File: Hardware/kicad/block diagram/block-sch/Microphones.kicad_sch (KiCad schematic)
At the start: 37 parts, among them J18 Conn_01x03, J19 Conn_01x03, J20 AudioJack3, K3 G6K-2, K4 G6K-2, Q3 BC817, U21 LM833D

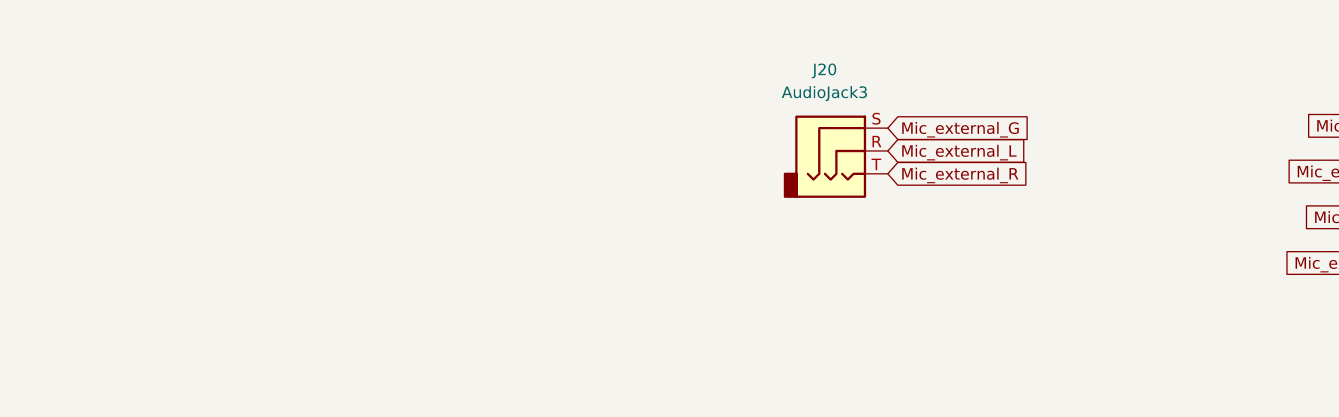
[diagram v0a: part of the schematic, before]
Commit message: new
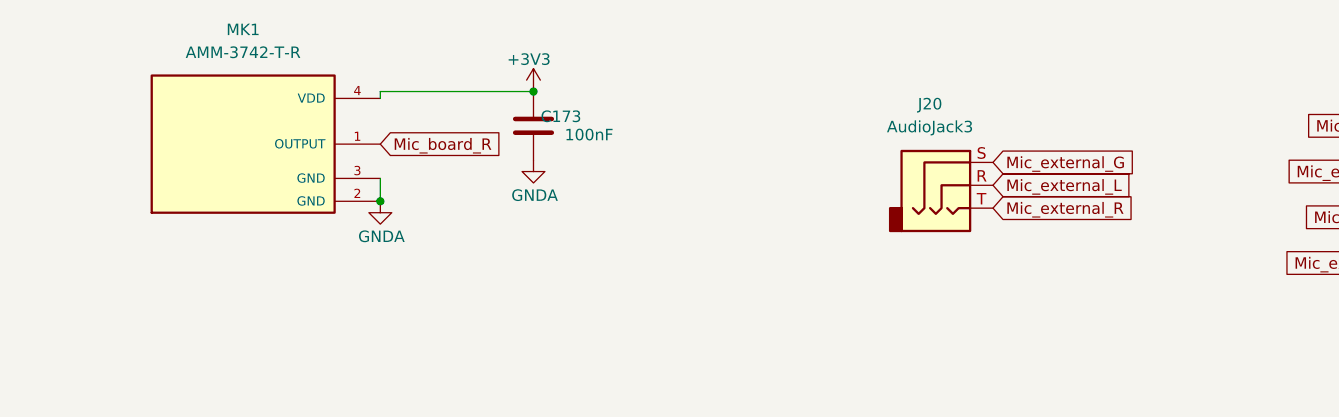
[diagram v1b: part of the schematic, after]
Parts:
- added C173: 100nF, Capacitor_SMD:C_1206_3216Metric, symbol Device:C
- added MK1: AMM-3742-T-R, amplituner_lib:MIC_AMM-3742-T-R, symbol amplituner_lib_sym:AMM-3742-T-R
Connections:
- net +3V3: now also C173.2, MK1.4 (VDD)
- net GNDA: now also C173.1, MK1.2 (GND), MK1.3 (GND)
- net Mic_board_R: now also MK1.1 (OUTPUT)
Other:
- moved on the sheet: J20
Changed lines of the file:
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@@
 (kicad_sch (version 20211123) (generator eeschema)
   (paper "A4")
+  (junction (at 73.66 25.908) (diameter 0) (color 0 0 0 0)
+  )
   (junction (at 37.338 139.446) (diameter 0) (color 0 0 0 0)
   )
@@
   (junction (at 108.458 81.788) (diameter 0) (color 0 0 0 0)
   )
+  (junction (at 56.642 38.1) (diameter 0) (color 0 0 0 0)
+  )
   (junction (at 69.342 128.524) (diameter 0) (color 0 0 0 0)
   )
@@
     (stroke (width 0) (type default) (color 0 0 0 0))
   )
+  (wire (pts (xy 56.642 25.908) (xy 56.642 26.67))
+    (stroke (width 0) (type default) (color 0 0 0 0))
+  )
   (wire (pts (xy 69.342 128.524) (xy 69.342 131.064))
     (stroke (width 0) (type default) (color 0 0 0 0))
@@
     (stroke (width 0) (type default) (color 0 0 0 0))
   )
+  (wire (pts (xy 73.66 25.908) (xy 56.642 25.908))
+    (stroke (width 0) (type default) (color 0 0 0 0))
+  )
   (wire (pts (xy 45.72 85.852) (xy 69.342 85.852))
     (stroke (width 0) (type default) (color 0 0 0 0))
@@
   )
   (wire (pts (xy 108.458 89.408) (xy 108.458 89.662))
+    (stroke (width 0) (type default) (color 0 0 0 0))
+  )
+  (wire (pts (xy 56.642 35.56) (xy 56.642 38.1))
     (stroke (width 0) (type default) (color 0 0 0 0))
   )
@@
     )
   )
-  (global_label "Mic_external_R" (shape input) (at 113.03 35.052 0) (fields_autoplaced)
+  (global_label "Mic_external_R" (shape input) (at 124.714 38.862 0) (fields_autoplaced)
     (effects (font (size 1.27 1.27)) (justify left))
-    (property "Intersheet References" "${INTERSHEET_REFS}" (id 0) (at 129.3847 34.9726 0)
+    (property "Intersheet References" "${INTERSHEET_REFS}" (id 0) (at 141.0687 38.7826 0)
       (effects (font (size 1.27 1.27)) (justify left) hide)
     )
@@
     )
   )
-  (global_label "Mic_external_L" (shape input) (at 113.03 32.512 0) (fields_autoplaced)
+  (global_label "Mic_external_L" (shape input) (at 124.714 36.322 0) (fields_autoplaced)
     (effects (font (size 1.27 1.27)) (justify left))
-    (property "Intersheet References" "${INTERSHEET_REFS}" (id 0) (at 129.1428 32.4326 0)
+    (property "Intersheet References" "${INTERSHEET_REFS}" (id 0) (at 140.8268 36.2426 0)
+      (effects (font (size 1.27 1.27)) (justify left) hide)
+    )
+  )
+  (global_label "Mic_board_R" (shape input) (at 56.642 31.75 0) (fields_autoplaced)
+    (effects (font (size 1.27 1.27)) (justify left))
+    (property "Intersheet References" "${INTERSHEET_REFS}" (id 0) (at 70.6986 31.8294 0)
       (effects (font (size 1.27 1.27)) (justify left) hide)
     )
@@
     )
   )
-  (global_label "Mic_external_G" (shape input) (at 113.03 29.972 0) (fields_autoplaced)
+  (global_label "Mic_external_G" (shape input) (at 124.714 33.782 0) (fields_autoplaced)
     (effects (font (size 1.27 1.27)) (justify left))
-    (property "Intersheet References" "${INTERSHEET_REFS}" (id 0) (at 129.3847 29.8926 0)
+    (property "Intersheet References" "${INTERSHEET_REFS}" (id 0) (at 141.0687 33.7026 0)
       (effects (font (size 1.27 1.27)) (justify left) hide)
     )
@@
     (pin "2")
   )
-  (symbol (lib_id "Connector:AudioJack3") (at 107.95 32.512 0) (unit 1)
-    (in_bom yes) (on_board yes) (fields_autoplaced)
-    (property "Reference" "J20" (id 0) (at 106.045 23.495 0))
-    (property "Value" "AudioJack3" (id 1) (at 106.045 26.035 0))
-    (property "Footprint" "Connector_Audio:Jack_3.5mm_CUI_SJ1-3533NG_Horizontal" (id 2) (at 107.95 32.512 0)
-      (effects (font (size 1.27 1.27)) hide)
-    )
-    (property "Datasheet" "~" (id 3) (at 107.95 32.512 0)
+  (symbol (lib_id "Connector:AudioJack3") (at 119.634 36.322 0) (unit 1)
+    (in_bom yes) (on_board yes) (fields_autoplaced)
+    (property "Reference" "J20" (id 0) (at 117.729 27.305 0))
+    (property "Value" "AudioJack3" (id 1) (at 117.729 29.845 0))
+    (property "Footprint" "Connector_Audio:Jack_3.5mm_CUI_SJ1-3533NG_Horizontal" (id 2) (at 119.634 36.322 0)
+      (effects (font (size 1.27 1.27)) hide)
+    )
+    (property "Datasheet" "~" (id 3) (at 119.634 36.322 0)
       (effects (font (size 1.27 1.27)) hide)
     )
@@
     (pin "2")
   )
+  (symbol (lib_id "power:+3V3") (at 73.66 25.908 0) (unit 1)
+    (in_bom yes) (on_board yes)
+    (property "Reference" "#PWR0167" (id 0) (at 73.66 29.718 0)
+      (effects (font (size 1.27 1.27)) hide)
+    )
+    (property "Value" "+3V3" (id 1) (at 73.152 22.352 0))
+    (property "Footprint" "" (id 2) (at 73.66 25.908 0)
+      (effects (font (size 1.27 1.27)) hide)
+    )
+    (property "Datasheet" "" (id 3) (at 73.66 25.908 0)
+      (effects (font (size 1.27 1.27)) hide)
+    )
+    (pin "1")
+  )
   (symbol (lib_id "Device:CP") (at 39.37 122.428 90) (unit 1)
     (in_bom yes) (on_board yes)
@@
     (pin "1")
     (pin "2")
+  )
+  (symbol (lib_id "power:GNDA") (at 56.642 38.1 0) (unit 1)
+    (in_bom yes) (on_board yes)
+    (property "Reference" "#PWR0166" (id 0) (at 56.642 44.45 0)
+      (effects (font (size 1.27 1.27)) hide)
+    )
+    (property "Value" "GNDA" (id 1) (at 56.769 42.037 0))
+    (property "Footprint" "" (id 2) (at 56.642 38.1 0)
+      (effects (font (size 1.27 1.27)) hide)
+    )
+    (property "Datasheet" "" (id 3) (at 56.642 38.1 0)
+      (effects (font (size 1.27 1.27)) hide)
+    )
+    (pin "1")
   )
   (symbol (lib_id "Relay:G6K-2") (at 250.952 42.164 90) (unit 1)
@@
     (pin "8")
   )
+  (symbol (lib_id "Device:C") (at 73.66 29.718 180) (unit 1)
+    (in_bom yes) (on_board yes)
+    (property "Reference" "C173" (id 0) (at 78.994 28.702 0)
+      (effects (font (size 1.27 1.27)) (justify left))
+    )
+    (property "Value" "100nF" (id 1) (at 82.55 30.734 0)
+      (effects (font (size 1.27 1.27)) (justify left))
+    )
+    (property "Footprint" "Capacitor_SMD:C_1206_3216Metric" (id 2) (at 72.6948 25.908 0)
+      (effects (font (size 1.27 1.27)) hide)
+    )
+    (property "Datasheet" "~" (id 3) (at 73.66 29.718 0)
+      (effects (font (size 1.27 1.27)) hide)
+    )
+    (pin "1")
+    (pin "2")
+  )
   (symbol (lib_id "Device:R") (at 247.142 75.438 270) (unit 1)
     (in_bom yes) (on_board yes)
@@
     (pin "1")
     (pin "2")
+  )
+  (symbol (lib_id "power:GNDA") (at 73.66 33.528 0) (unit 1)
+    (in_bom yes) (on_board yes)
+    (property "Reference" "#PWR0168" (id 0) (at 73.66 39.878 0)
+      (effects (font (size 1.27 1.27)) hide)
+    )
+    (property "Value" "GNDA" (id 1) (at 73.787 37.465 0))
+    (property "Footprint" "" (id 2) (at 73.66 33.528 0)
+      (effects (font (size 1.27 1.27)) hide)
+    )
+    (property "Datasheet" "" (id 3) (at 73.66 33.528 0)
+      (effects (font (size 1.27 1.27)) hide)
+    )
+    (pin "1")
   )
   (symbol (lib_id "Device:R") (at 41.148 139.446 270) (unit 1)
@@
     (pin "1")
   )
+  (symbol (lib_id "amplituner_lib_sym:AMM-3742-T-R") (at 41.402 31.75 0) (unit 1)
+    (in_bom yes) (on_board yes) (fields_autoplaced)
+    (property "Reference" "MK1" (id 0) (at 41.402 19.05 0))
+    (property "Value" "AMM-3742-T-R" (id 1) (at 41.402 21.59 0))
+    (property "Footprint" "amplituner_lib:MIC_AMM-3742-T-R" (id 2) (at 35.052 20.32 0)
+      (effects (font (size 1.27 1.27)) (justify left bottom) hide)
+    )
+    (property "Datasheet" "" (id 3) (at 41.402 31.75 0)
+      (effects (font (size 1.27 1.27)) (justify left bottom) hide)
+    )
+    (property "STANDARD" "Manufacturer Recommendations" (id 4) (at 35.052 22.86 0)
+      (effects (font (size 1.27 1.27)) (justify left bottom) hide)
+    )
+    (property "MAXIMUM_PACKAGE_HEIGHT" "1.3 mm" (id 5) (at 35.052 17.78 0)
+      (effects (font (size 1.27 1.27)) (justify left bottom) hide)
+    )
+    (property "MANUFACTURER" "PUI AUDIO" (id 6) (at 35.052 15.24 0)
+      (effects (font (size 1.27 1.27)) (justify left bottom) hide)
+    )
+    (property "PARTREV" "10/12/2020" (id 7) (at 43.942 17.78 0)
+      (effects (font (size 1.27 1.27)) (justify left bottom) hide)
+    )
+    (pin "1")
+    (pin "2")
+    (pin "3")
+    (pin "4")
+  )
   (symbol (lib_id "Device:R") (at 30.48 106.426 180) (unit 1)
